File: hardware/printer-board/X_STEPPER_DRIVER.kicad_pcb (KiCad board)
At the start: 2 copper layers, 7 parts, among them J3 MS_SELECT, J4 TO_MOTOR, U3 A4988_MODULE

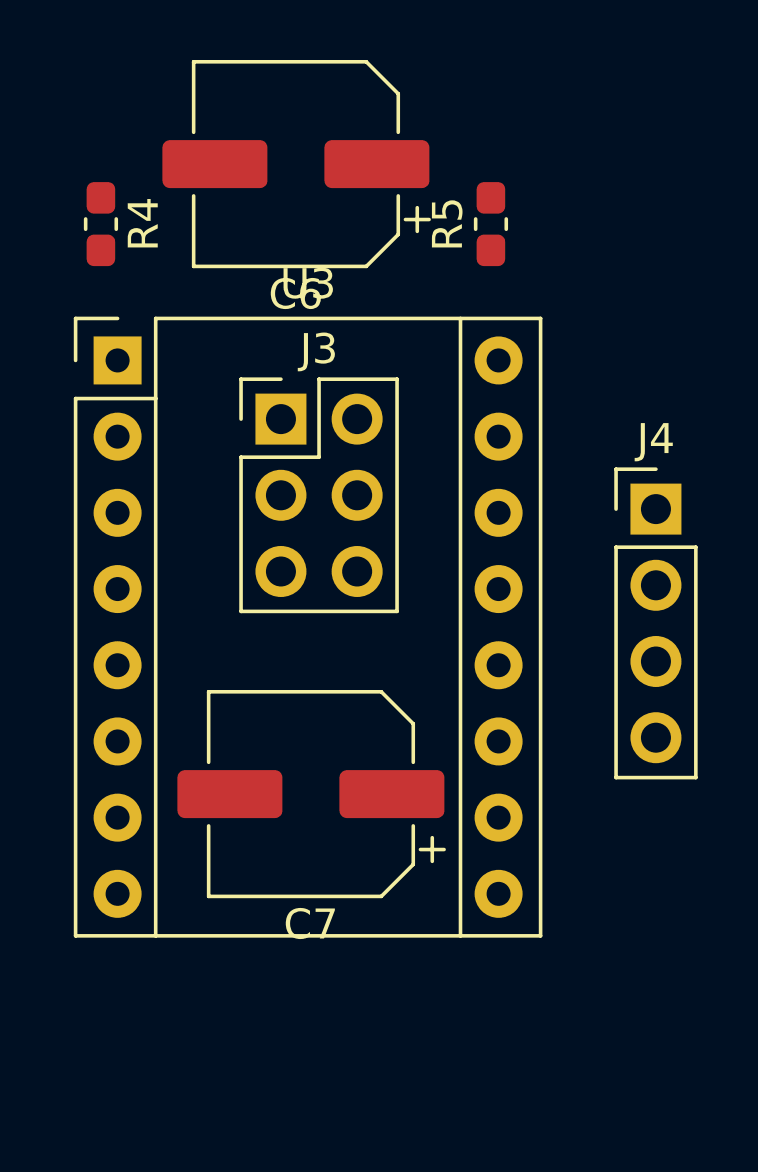
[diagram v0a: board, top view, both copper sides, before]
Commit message: update,
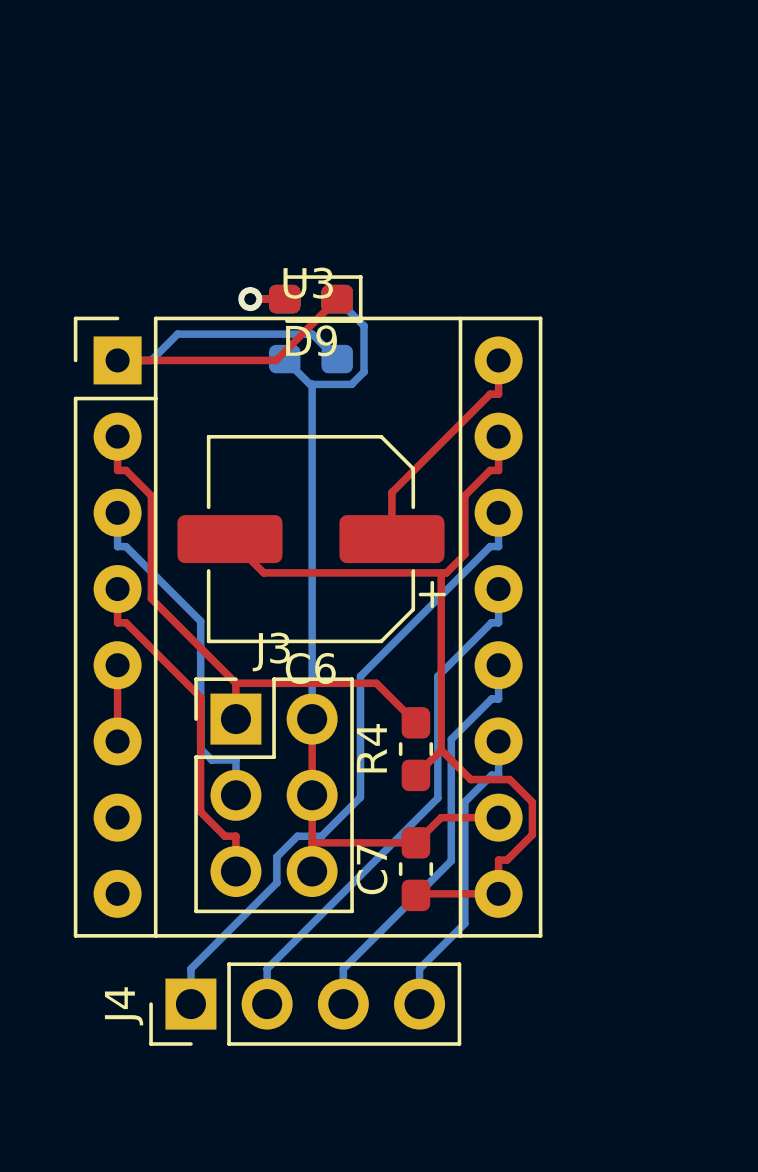
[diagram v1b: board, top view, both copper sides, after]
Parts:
- removed R5: R103,0603, Resistor_SMD:R_0603_1608Metric_Pad1.05x0.95mm_HandSolder
- added D9: LED_BLUE,0603, LED_SMD:LED_0603_1608Metric_Pad1.05x0.95mm_HandSolder, F.Cu at (83.0, 44.5)
- added R11: R102,0603, Resistor_SMD:R_0603_1608Metric_Pad1.05x0.95mm_HandSolder, B.Cu at (83.0, 44.5)
- added R13: R103,0603, Resistor_SMD:R_0603_1608Metric_Pad1.05x0.95mm_HandSolder, B.Cu at (83.0, 46.5)
- C7: value CP100uf,25V -> C104,0603; footprint Capacitor_SMD:CP_Elec_6.3x7.7 -> Capacitor_SMD:C_0603_1608Metric_Pad1.05x0.95mm_HandSolder
- J4: value TO_MOTOR -> X
- moved J4 22.6 mm to (79.0, 68.0), turned to 90 degrees
- moved R4 20.4 mm to (86.5, 59.5), turned to 90 degrees
- moved C6 12.5 mm to (83.0, 52.5)
- moved J3 10.1 mm to (80.5, 58.5)
- moved C7 4.30 mm to (86.5, 63.5), turned to 90 degrees
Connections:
- net /DIR renamed /X_DIR
- net /STEP renamed /X_STEP
- C7 pad 1: +5V -> GND
- C7 pad 2: GND -> +3V3_STM32
- J3 pad 2: +5V -> +3V3_STM32
- J3 pad 4: +5V -> +3V3_STM32
- J3 pad 6: +5V -> +3V3_STM32
- U3 pad 1: /~EN~ -> /~X_EN~
- U3 pad 10: +5V -> +3V3_STM32
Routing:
- net GND: track 0.00 -> 30.4 mm
- net +3V3_STM32: track 0.00 -> 28.8 mm
- net Net-(J4-Pad1): track 0.00 -> 21.3 mm
- net Net-(J3-Pad1): track 0.00 -> 17.8 mm
- net Net-(J4-Pad2): track 0.00 -> 17.2 mm
- net /~X_EN~: track 0.00 -> 16.2 mm
- net Net-(J4-Pad3): track 0.00 -> 13.6 mm
- net Net-(J3-Pad3): track 0.00 -> 11.7 mm
- net Net-(J3-Pad5): track 0.00 -> 11.4 mm
- net Net-(J4-Pad4): track 0.00 -> 9.98 mm
- net +12V: track 0.00 -> 7.59 mm
- net Net-(U3-Pad5): track 0.00 -> 2.54 mm
- net Net-(D9-Pad2): track 0.00 -> 2.29 mm, vias 0 -> 1

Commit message: update heater layouts,
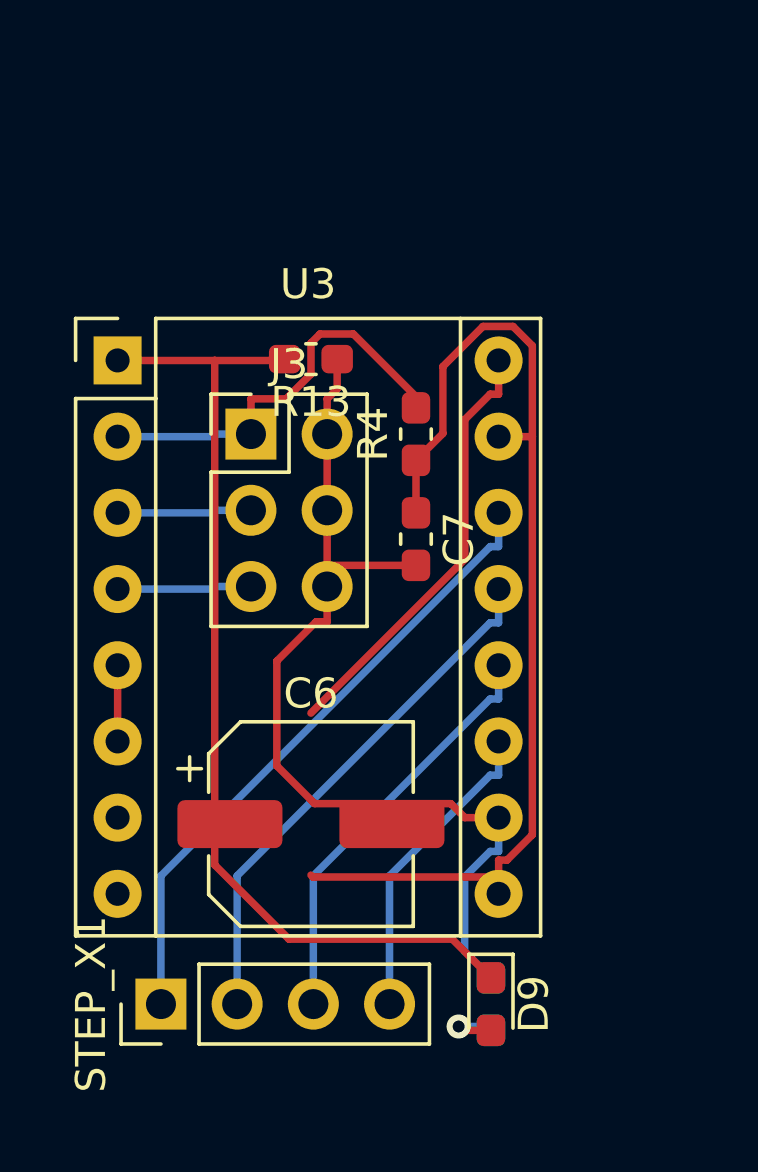
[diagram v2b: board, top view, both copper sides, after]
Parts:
- removed J4: X, Connector_PinHeader_2.54mm:PinHeader_1x04_P2.54mm_Vertical
- added STEP_X1: X, Connector_PinHeader_2.54mm:PinHeader_1x04_P2.54mm_Vertical, F.Cu at (78.0, 68.0)
- R13: moved to F.Cu
- moved D9 24.3 mm to (89.0, 68.0), turned to 270 degrees
- moved R11 24.3 mm to (89.0, 68.0), turned to 270 degrees
- moved C7 11.0 mm to (86.5, 52.5), turned to 270 degrees
- moved R4 10.5 mm to (86.5, 49.0)
- moved J3 9.51 mm to (81.0, 49.0)
- moved C6 9.50 mm to (83.0, 62.0), turned to 0 degrees
- turned R13 to 180 degrees
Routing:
- net /~X_EN~: track 16.2 -> 33.2 mm
- net Net-(J3-Pad3): track 11.7 -> 4.48 mm
- net Net-(J3-Pad5): track 11.4 -> 4.48 mm
- net +12V: track 7.59 -> 14.5 mm
- net GND: track 30.4 -> 35.4 mm
- net Net-(J3-Pad1): track 17.8 -> 13.9 mm
- net +3V3_STM32: track 28.8 -> 32.0 mm
